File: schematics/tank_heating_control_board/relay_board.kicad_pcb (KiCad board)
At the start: 2 copper layers, 45 x 75 mm, 51 parts, among them J1 Programming Header, P1 ACT_PWR, P2 ACT_PWR, P3 ACTUATOR, Q1 MMBF170, Q2 MMBF170, SW1 SW_DIP_x04, U1 SPST_POWER_RELAY, U2 PIC16F1826-ISO, U3 dpdt_relay, U4 INA180A1, U5 CONN_01x05, U6 INA180A1, U7 CONN_01x05

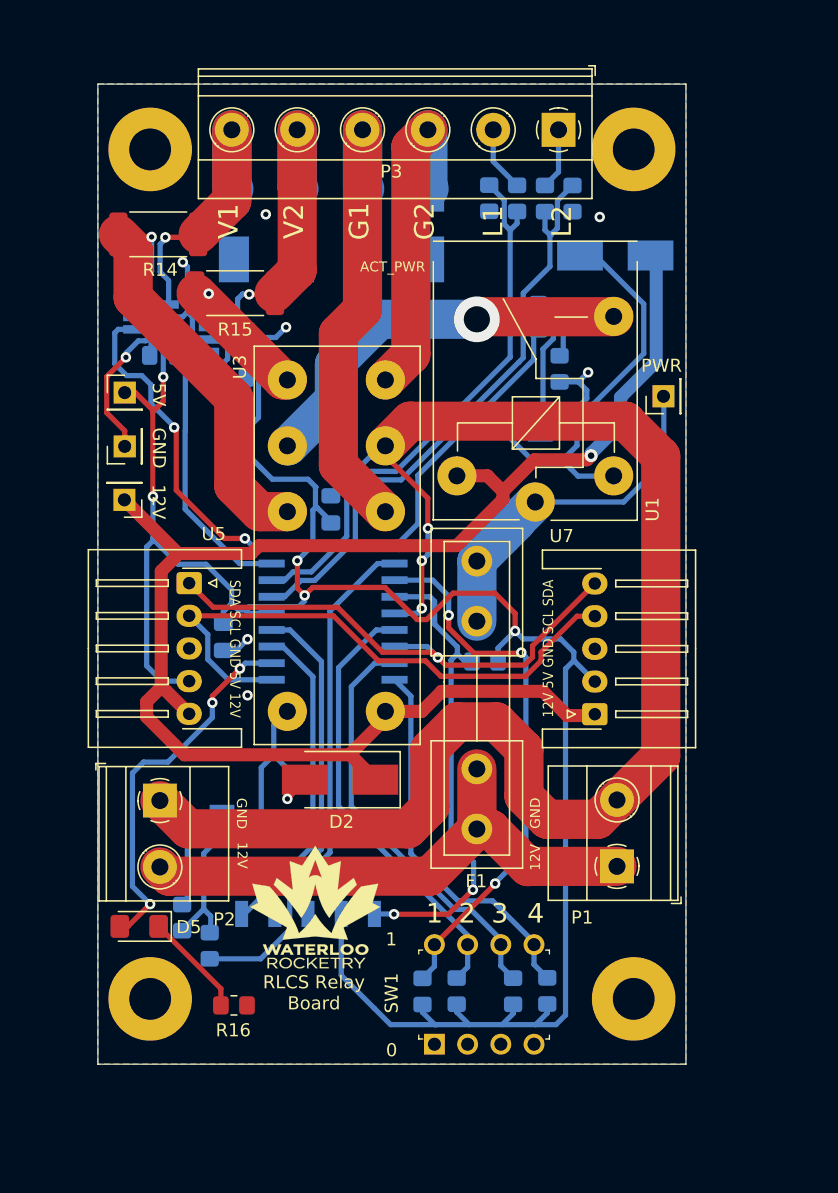
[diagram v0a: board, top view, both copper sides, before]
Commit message: routed
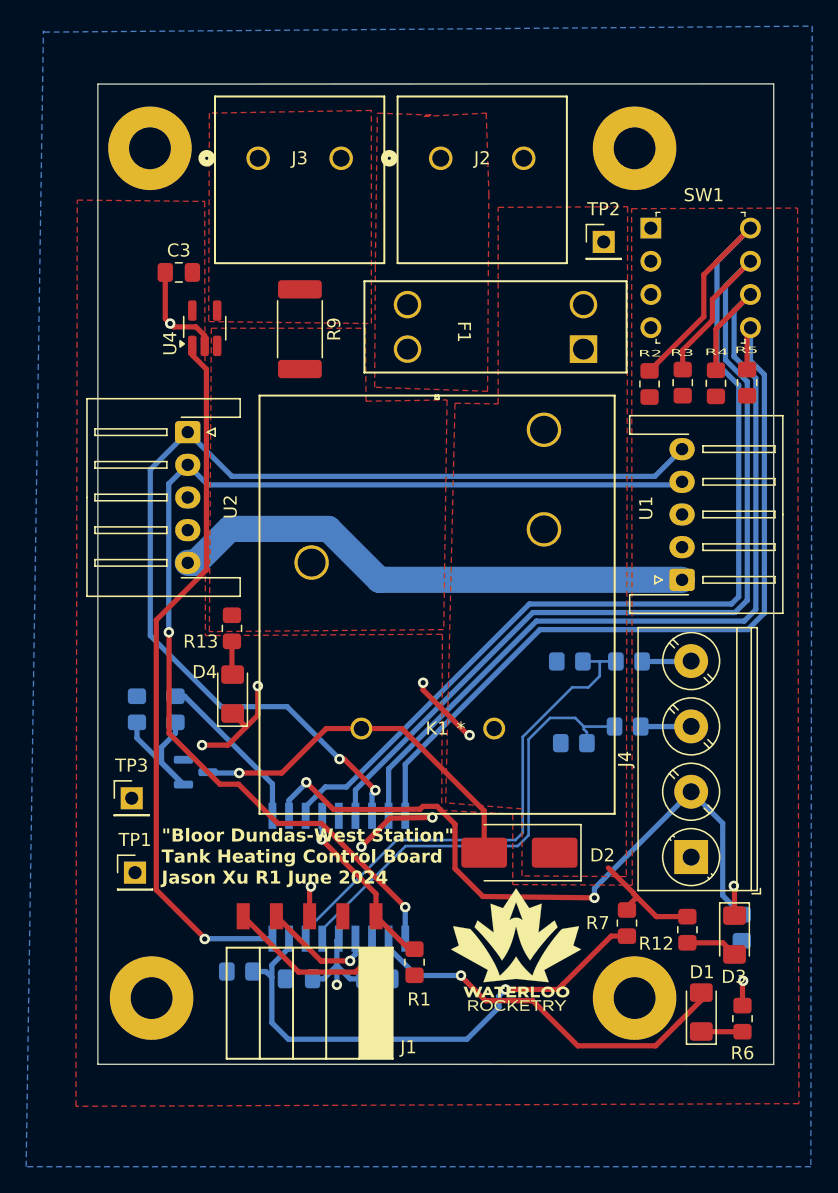
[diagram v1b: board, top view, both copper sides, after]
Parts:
- removed ? (x4): MountingHole_3.2mm_M3_Pad, MountingHole:MountingHole_3.2mm_M3_Pad
- removed C4: 0.1uF, Capacitor_SMD:C_0805_2012Metric_Pad1.18x1.45mm_HandSolder
- removed D5: BLUE 3.2V 10mA, LED_SMD:LED_1206_3216Metric_Pad1.42x1.75mm_HandSolder
- removed D6, D7: D, Diode_SMD:D_SMB_Handsoldering
- removed the G*** at (146.6, 132.0)
- removed P1, P2: ACT_PWR, TerminalBlock_Phoenix:TerminalBlock_Phoenix_MKDS-1,5-2-5.08_1x02_P5.08mm_Horizontal
- removed P3: ACTUATOR, TerminalBlock_Phoenix:TerminalBlock_Phoenix_MKDS-1,5-6_1x06_P5.00mm_Horizontal
- removed Q2: MMBF170, Package_TO_SOT_SMD:SOT-23_Handsoldering
- removed TP0: TEST_1P, custom:Socket_Strip_Straight_1x01_Pitch2.54mm
- removed U5, U7: CONN_01x05, Connector_JST:JST_XH_S5B-XH-A-1_1x05_P2.50mm_Horizontal
- removed U6: INA180A1, Package_TO_SOT_SMD:SOT-23-5_HandSoldering
- added G***: LOGO, custom:rocketry_logo_small, F.Cu at (162.0, 135.2)
- added J2: Power IN from battery, custom:CONN_1714955_PXC, F.Cu at (156.2, 74.7)
- added J3: Power OUT to heater, custom:CONN_1714955_PXC, F.Cu at (142.3, 74.7)
- added J4: Vsense and Thermistor, TerminalBlock_Phoenix:TerminalBlock_Phoenix_PT-1,5-4-5.0-H_1x04_P5.00mm_Horizontal, F.Cu at (175.4, 128.2)
- added K1: AZ2150-1AE-24DEF, custom:AZ2150_AMZ, F.Cu at (160.3, 118.3)
- added R17: 60.4K 1%, Resistor_SMD:R_0805_2012Metric_Pad1.20x1.40mm_HandSolder, B.Cu at (170.5, 118.2)
- added R18: 10K 1%, Resistor_SMD:R_0805_2012Metric_Pad1.20x1.40mm_HandSolder, B.Cu at (166.4, 119.4)
- added REF**: MountingHole_3.2mm_M3_Pad, MountingHole:MountingHole_3.2mm_M3_Pad, F.Cu at (171.1, 138.9)
- added REF**: MountingHole_3.2mm_M3_Pad, MountingHole:MountingHole_3.2mm_M3_Pad, F.Cu at (134.0, 73.9)
- added REF**: MountingHole_3.2mm_M3_Pad, MountingHole:MountingHole_3.2mm_M3_Pad, F.Cu at (134.1, 138.9)
- added REF**: MountingHole_3.2mm_M3_Pad, MountingHole:MountingHole_3.2mm_M3_Pad, F.Cu at (171.1, 73.9)
- C3, R2, R3, R4, U4: moved to F.Cu
- D1: value D -> BLUE 3.2V 10mA; footprint Diode_SMD:D_SMB_Handsoldering -> LED_SMD:LED_1206_3216Metric_Pad1.42x1.75mm_HandSolder; moved to F.Cu
- D2: value D -> STPS2L25U
- D3: value D -> RED; footprint Diode_SMD:D_SMB_Handsoldering -> LED_SMD:LED_1206_3216Metric_Pad1.42x1.75mm_HandSolder; moved to F.Cu
- D4: value D -> GREEN; footprint Diode_SMD:D_SMB_Handsoldering -> LED_SMD:LED_1206_3216Metric_Pad1.42x1.75mm_HandSolder; moved to F.Cu
- F1: value FUSE -> 30A; footprint custom:littlefuse_01000020Z -> custom:3557-10_KEY
- J1: value Programming Header -> Conn_01x05_Socket; moved to F.Cu
- Q1: footprint Package_TO_SOT_SMD:SOT-23_Handsoldering -> Package_TO_SOT_SMD:SOT-23
- R1: value 10k -> 10K; moved to F.Cu
- R10: value 10K -> 150
- R12, R13: value 10K -> 2.2K; moved to F.Cu
- R14: value 0.01 -> TBD; footprint Resistor_SMD:R_2512_6332Metric_Pad1.40x3.35mm_HandSolder -> Resistor_SMD:R_0805_2012Metric_Pad1.20x1.40mm_HandSolder; moved to B.Cu
- R15: value 0.01 -> 60.4K 1%; footprint Resistor_SMD:R_2512_6332Metric_Pad1.40x3.35mm_HandSolder -> Resistor_SMD:R_0805_2012Metric_Pad1.20x1.40mm_HandSolder; moved to B.Cu
- R16: value 180 -> 10K 1%; moved to B.Cu
- R5: value 150 -> 10k; moved to F.Cu
- R6: value 150 -> 180; moved to F.Cu
- R7: value 20K -> 60.4K 1%; moved to F.Cu
- R8: value 10K -> 10K 1%
- R9: value 20K -> 0.001 1%; footprint Resistor_SMD:R_0805_2012Metric_Pad1.20x1.40mm_HandSolder -> Resistor_SMD:R_2512_6332Metric_Pad1.40x3.35mm_HandSolder; moved to F.Cu
- U1: value SPST_POWER_RELAY -> JST I2C Connector; footprint custom:Relay_SPST_G5LE-1A -> Connector_JST:JST_XH_S5B-XH-A-1_1x05_P2.50mm_Horizontal
- U2: value PIC16F1826-ISO -> JST I2C Connector; footprint custom:PIC16F1826-ISO -> Connector_JST:JST_XH_S5B-XH-A-1_1x05_P2.50mm_Horizontal; moved to F.Cu
- U3: value dpdt_relay -> PIC16F1826-ISO; footprint custom:Relay_DPDT_RT424012F -> custom:PIC16F1826-ISO; moved to B.Cu
- moved R14 69.3 mm to (179.3, 133.6), turned to -90 degrees
- moved SW1 64.6 mm to (172.3, 80.0), turned to 0 degrees
- moved R8 62.2 mm to (140.9, 136.9), turned to 180 degrees
- moved D3 61.3 mm to (178.7, 134.1)
- moved D1 58.3 mm to (176.2, 140.0), turned to 90 degrees
- moved R7 56.1 mm to (170.5, 133.2)
- moved TP3 51.0 mm to (132.6, 123.6), turned to 0 degrees
- moved R10 49.5 mm to (135.9, 116.8), turned to 90 degrees
- moved R2 48.7 mm to (172.2, 91.9)
- moved R3 48.3 mm to (174.8, 91.8)
- moved R4 48.2 mm to (177.3, 91.9)
- moved C2 47.3 mm to (151.4, 137.5), turned to 180 degrees
- moved R11 41.5 mm to (133.0, 116.8), turned to 90 degrees
- moved R15 41.3 mm to (170.6, 113.2)
- moved R6 41.1 mm to (179.3, 140.5), turned to 90 degrees
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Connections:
- D1 pad 1: +12V -> Net-(D1-K)
- D1 pad 2: Net-(D1-Pad2) -> Net-(D1-A)
- D2 pad 1: +12V -> +24V
- D2 pad 2: Net-(D2-Pad2) -> Net-(D2-A)
- D3 pad 1: /G1 -> GND
- D3 pad 2: GND -> Net-(D3-A)
- D4 pad 1: /G2 -> GND
- D4 pad 2: GND -> Net-(D4-A)
- F1 pad 1: Net-(F1-Pad1) -> +24V
- F1 pad 2: Net-(F1-Pad2) -> Net-(J2-Pin_1)
- J1 pad 1: /ICSPCLK -> /~{MCLR}
- J1 pad 2: /ICSPDAT -> +5V
- J1 pad 4: +5V -> /ICSPDAT
- J1 pad 5: /~{MCLR} -> /ICSPCLK
- Q1 pad 1: Net-(Q1-Pad1) -> Net-(Q1-G)
- Q1 pad 3: Net-(D1-Pad2) -> Net-(D2-A)
- R1 pad 2: /DIP_1 -> /~{MCLR}
- R10 pad 1: /LIM2 -> Net-(Q1-G)
- R10 pad 2: GND -> /PWR_CTRL
- R11 pad 1: Net-(Q1-Pad1) -> Net-(Q1-G)
- R12 pad 1: Net-(Q2-Pad1) -> +24V
- R12 pad 2: GND -> Net-(D3-A)
- R13 pad 1: +5V -> /PWR_OUT
- R13 pad 2: /~{MCLR} -> Net-(D4-A)
- R14 pad 1: /P1 -> /THERMISTOR
- R14 pad 2: Net-(R14-Pad2) -> GND
- R15 pad 1: /P2 -> Net-(J4-Pin_4)
- R15 pad 2: Net-(R15-Pad2) -> /HEATER_VSENSE_P
- R16 pad 1: Net-(D5-Pad1) -> /HEATER_VSENSE_P
- R2 pad 2: /DIP_2 -> /DIP_1
- R3 pad 2: /DIP_3 -> /DIP_2
- R4 pad 2: /DIP_4 -> /DIP_3
- R5 pad 1: Net-(Q1-Pad1) -> +5V
- R5 pad 2: /POWER -> /DIP_4
- R6 pad 1: Net-(Q2-Pad1) -> Net-(D1-K)
- R6 pad 2: /SELECT -> GND
- R7 pad 1: Net-(P3-Pad2) -> +24V
- R7 pad 2: /LIM1 -> /24VSENSE
- R8 pad 1: /LIM1 -> /24VSENSE
- R9 pad 1: Net-(P3-Pad1) -> Net-(J3-Pin_1)
- R9 pad 2: /LIM2 -> /PWR_OUT
- TP1 pad 1: +12V -> GND
- TP2 pad 1: +5V -> +24V
- TP3 pad 1: Net-(F1-Pad2) -> +5V
- U1 pad 1: +12V -> Net-(U1-Pad1)
- U1 pad 2: Net-(D1-Pad2) -> +5V
- U1 pad 3: Net-(F1-Pad2) -> GND
- U1 pad 4: Net-(U1-Pad4) -> /SCL
- U2 pad 1: /POWER -> /SDA
- U2 pad 2: /SELECT -> /SCL
- U2 pad 3: /DIP_1 -> GND
- U2 pad 4: /~{MCLR} -> +5V
- U2 pad 5: GND -> Net-(U1-Pad1)
- U3 pad 1: Net-(U1-Pad4) -> /PWR_CTRL
- U3 pad 2: GND -> /THERMISTOR
- U3 pad 3: Net-(D2-Pad2) -> /DIP_1
- U3 pad 4: +12V -> /~{MCLR}
- U3 pad 5: Net-(R14-Pad2) -> GND
- U3 pad 6: Net-(R15-Pad2) -> /DIP_2
- U3 pad 7: /G1 -> /SDA
- U3 pad 8: /G2 -> /DIP_3
- U4 pad 1: /CURR_SENSE_1 -> /CURR_SENSE
- U4 pad 3: Net-(R14-Pad2) -> /PWR_OUT
- U4 pad 4: /P1 -> Net-(J3-Pin_1)
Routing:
- net +5V: track 172.8 -> 8.35 mm, vias 5 -> 1
- net GND: track 175.7 -> 36.0 mm, vias 11 -> 10
- net +12V: track 120.1 -> 0.00 mm, vias 1 -> 0
- net /CURR_SENSE: track 0.00 -> 54.3 mm, vias 0 -> 1
- net /THERMISTOR: track 0.00 -> 53.5 mm, vias 0 -> 2
- net /LIM2: track 45.5 -> 0.00 mm
- net /DIP_1: track 41.8 -> 84.6 mm, vias 3 -> 0
- net /LIM1: track 42.6 -> 0.00 mm
- net Net-(F1-Pad1): track 42.6 -> 0.00 mm
- net /SDA: track 39.5 -> 81.8 mm, vias 1 -> 2
- net /DIP_2: track 33.7 -> 75.8 mm
- net /SCL: track 44.7 -> 85.7 mm, vias 0 -> 2
- net /24VSENSE: track 0.00 -> 41.0 mm, vias 0 -> 1
- net Net-(U1-Pad1): track 0.00 -> 40.5 mm
- net /HEATER_VSENSE_P: track 0.00 -> 39.8 mm
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- added copper zone on F.Cu, net +24V
- added copper zone on F.Cu, net +5V
- added copper zone on F.Cu, net /PWR_OUT
- added copper zone on F.Cu, net Net-(J2-Pin_1)
- added copper zone on F.Cu, net Net-(J3-Pin_1)
- removed copper zone on F.Cu, net GND
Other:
- board size 45 x 75 mm -> 51.7 x 75 mm
- board text added: "{dblquote}Bloor Dundas-West Station{dblquote} Tank Heating Control Board Jason Xu R1 June 2024"
- board text removed: "0"
- board text removed: "1"
- board text removed: "12V"
- board text removed: "12V 5V GND SCL SDA"
- board text removed: "2"
- board text removed: "3"
- board text removed: "4"
- board text removed: "5V"
- board text removed: "ACT_PWR"
- board text removed: "G1"
- board text removed: "G2"
- board text removed: "GND"
- board text removed: "L1"
- board text removed: "L2"
- board text removed: "PWR"
- board text removed: "RLCS Relay Board"
- board text removed: "SDA SCL GND 5V 12V"
- board text removed: "V1"
- board text removed: "V2"
- board text removed: "~{MCLR} 5V"
